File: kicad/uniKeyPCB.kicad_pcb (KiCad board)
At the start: 2 copper layers, 94 x 94 mm, 160 parts, among them J1 Conn_01x03_Socket, J2 Conn_01x03_Socket, J3 Conn_01x03_Socket, J4 Conn_01x03_Socket, J5 Conn_01x02_Socket, J6 Conn_01x02_Socket, J7 Conn_01x02_Socket, J8 Conn_01x02_Socket, SW1 SW_CHOC_HS, SW2 SW_MX_HS

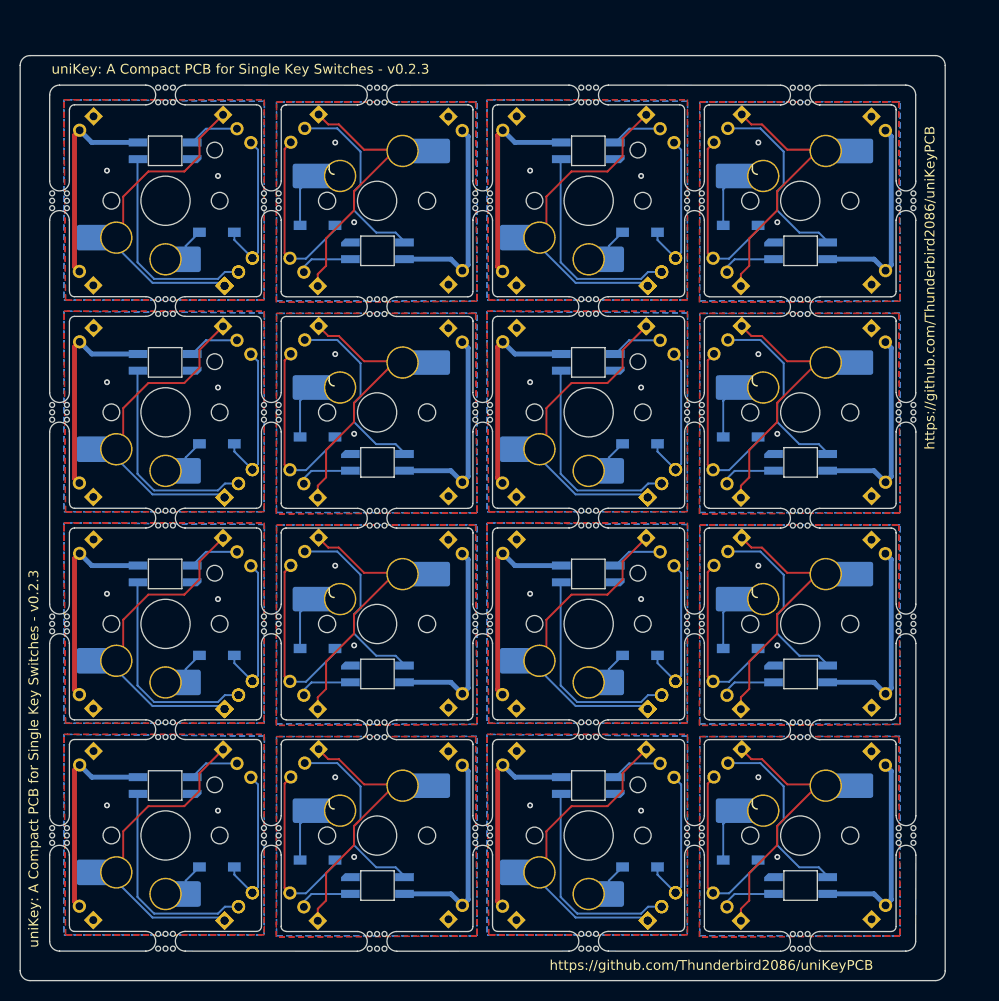
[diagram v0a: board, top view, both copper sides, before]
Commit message: more connectors
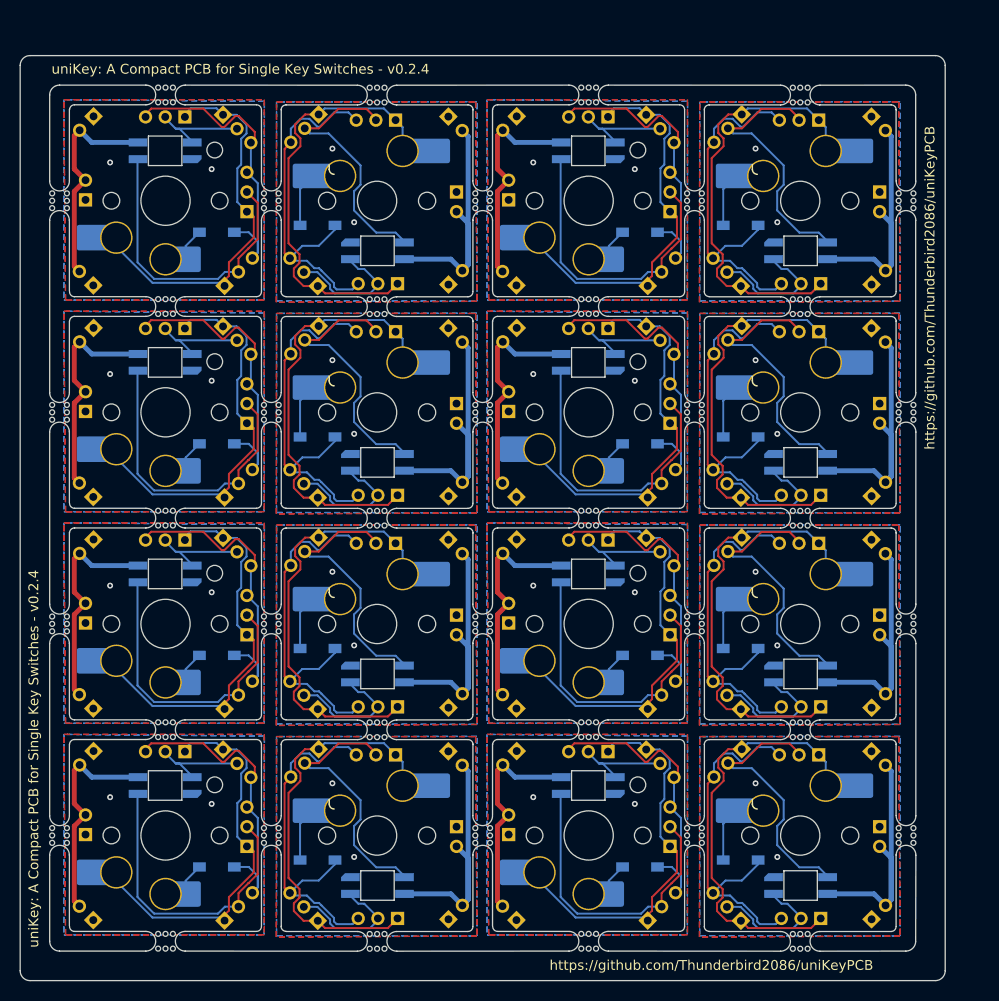
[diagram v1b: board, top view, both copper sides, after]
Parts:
- removed the J2 at (76.3, 136.0) (x2)
- removed the J2 at (119.3, 71.5) (x2)
- removed the J2 at (119.3, 114.5) (x2)
- removed the J2 at (76.3, 114.5) (x2)
- removed the J2 at (119.3, 136.0) (x2)
- removed the J2 at (76.3, 93.0) (x2)
- removed the J2 at (76.3, 71.5)
- removed the J2 at (119.3, 93.0) (x2)
- added J10: Conn_01x03_Socket, Connector_PinHeader_2.00mm:PinHeader_1x03_P2.00mm_Vertical, B.Cu at (121.6, 85.5)
- added J10: Conn_01x03_Socket, Connector_PinHeader_2.00mm:PinHeader_1x03_P2.00mm_Vertical, B.Cu at (121.6, 128.5)
- added J10: Conn_01x03_Socket, Connector_PinHeader_2.00mm:PinHeader_1x03_P2.00mm_Vertical, B.Cu at (78.6, 64.0)
- added J10: Conn_01x03_Socket, Connector_PinHeader_2.00mm:PinHeader_1x03_P2.00mm_Vertical, B.Cu at (78.6, 107.0)
- added J10: Conn_01x03_Socket, Connector_PinHeader_2.00mm:PinHeader_1x03_P2.00mm_Vertical, B.Cu at (121.6, 107.0)
- added J10: Conn_01x03_Socket, Connector_PinHeader_2.00mm:PinHeader_1x03_P2.00mm_Vertical, B.Cu at (78.6, 85.5)
- added J10: Conn_01x03_Socket, Connector_PinHeader_2.00mm:PinHeader_1x03_P2.00mm_Vertical, B.Cu at (121.6, 64.0)
- added J10: Conn_01x03_Socket, Connector_PinHeader_2.00mm:PinHeader_1x03_P2.00mm_Vertical, B.Cu at (78.6, 128.5)
- added J11: Conn_01x03_Socket, Connector_PinHeader_2.00mm:PinHeader_1x03_P2.00mm_Vertical, B.Cu at (93.9, 92.8)
- added J11: Conn_01x03_Socket, Connector_PinHeader_2.00mm:PinHeader_1x03_P2.00mm_Vertical, B.Cu at (93.9, 114.3)
- added J11: Conn_01x03_Socket, Connector_PinHeader_2.00mm:PinHeader_1x03_P2.00mm_Vertical, B.Cu at (136.9, 135.8)
- added J11: Conn_01x03_Socket, Connector_PinHeader_2.00mm:PinHeader_1x03_P2.00mm_Vertical, B.Cu at (136.9, 92.8)
- added J11: Conn_01x03_Socket, Connector_PinHeader_2.00mm:PinHeader_1x03_P2.00mm_Vertical, B.Cu at (93.9, 71.3)
- added J11: Conn_01x03_Socket, Connector_PinHeader_2.00mm:PinHeader_1x03_P2.00mm_Vertical, B.Cu at (93.9, 135.8)
- added J11: Conn_01x03_Socket, Connector_PinHeader_2.00mm:PinHeader_1x03_P2.00mm_Vertical, B.Cu at (136.9, 71.3)
- added J11: Conn_01x03_Socket, Connector_PinHeader_2.00mm:PinHeader_1x03_P2.00mm_Vertical, B.Cu at (136.9, 114.3)
- added J12: Conn_01x03_Socket, Connector_PinHeader_2.00mm:PinHeader_1x03_P2.00mm_Vertical, B.Cu at (93.7, 76.2)
- added J12: Conn_01x03_Socket, Connector_PinHeader_2.00mm:PinHeader_1x03_P2.00mm_Vertical, B.Cu at (93.7, 54.7)
- added J12: Conn_01x03_Socket, Connector_PinHeader_2.00mm:PinHeader_1x03_P2.00mm_Vertical, B.Cu at (136.7, 119.2)
- added J12: Conn_01x03_Socket, Connector_PinHeader_2.00mm:PinHeader_1x03_P2.00mm_Vertical, B.Cu at (136.7, 76.2)
- added J12: Conn_01x03_Socket, Connector_PinHeader_2.00mm:PinHeader_1x03_P2.00mm_Vertical, B.Cu at (93.7, 119.2)
- added J12: Conn_01x03_Socket, Connector_PinHeader_2.00mm:PinHeader_1x03_P2.00mm_Vertical, B.Cu at (93.7, 97.7)
- added J12: Conn_01x03_Socket, Connector_PinHeader_2.00mm:PinHeader_1x03_P2.00mm_Vertical, B.Cu at (136.7, 97.7)
- added J12: Conn_01x03_Socket, Connector_PinHeader_2.00mm:PinHeader_1x03_P2.00mm_Vertical, B.Cu at (136.7, 54.7)
- added J13: Conn_01x02_Socket, Connector_PinSocket_2.00mm:PinSocket_1x02_P2.00mm_Vertical, B.Cu at (142.9, 126.5)
- added J13: Conn_01x02_Socket, Connector_PinSocket_2.00mm:PinSocket_1x02_P2.00mm_Vertical, B.Cu at (99.9, 62.0)
- added J13: Conn_01x02_Socket, Connector_PinSocket_2.00mm:PinSocket_1x02_P2.00mm_Vertical, B.Cu at (99.9, 83.5)
- added J13: Conn_01x02_Socket, Connector_PinSocket_2.00mm:PinSocket_1x02_P2.00mm_Vertical, B.Cu at (142.9, 105.0)
- added J13: Conn_01x02_Socket, Connector_PinSocket_2.00mm:PinSocket_1x02_P2.00mm_Vertical, B.Cu at (142.9, 62.0)
- added J13: Conn_01x02_Socket, Connector_PinSocket_2.00mm:PinSocket_1x02_P2.00mm_Vertical, B.Cu at (99.9, 126.5)
- added J13: Conn_01x02_Socket, Connector_PinSocket_2.00mm:PinSocket_1x02_P2.00mm_Vertical, B.Cu at (99.9, 105.0)
- added J13: Conn_01x02_Socket, Connector_PinSocket_2.00mm:PinSocket_1x02_P2.00mm_Vertical, B.Cu at (142.9, 83.5)
- added J14: Conn_01x02_Socket, Connector_PinSocket_2.00mm:PinSocket_1x02_P2.00mm_Vertical, B.Cu at (62.2, 105.8)
- added J14: Conn_01x02_Socket, Connector_PinSocket_2.00mm:PinSocket_1x02_P2.00mm_Vertical, B.Cu at (105.2, 84.3)
- added J14: Conn_01x02_Socket, Connector_PinSocket_2.00mm:PinSocket_1x02_P2.00mm_Vertical, B.Cu at (105.2, 105.8)
- added J14: Conn_01x02_Socket, Connector_PinSocket_2.00mm:PinSocket_1x02_P2.00mm_Vertical, B.Cu at (62.2, 84.3)
- added J14: Conn_01x02_Socket, Connector_PinSocket_2.00mm:PinSocket_1x02_P2.00mm_Vertical, B.Cu at (105.2, 127.3)
- added J14: Conn_01x02_Socket, Connector_PinSocket_2.00mm:PinSocket_1x02_P2.00mm_Vertical, B.Cu at (105.2, 62.8)
- added J14: Conn_01x02_Socket, Connector_PinSocket_2.00mm:PinSocket_1x02_P2.00mm_Vertical, B.Cu at (62.2, 62.8)
- added J14: Conn_01x02_Socket, Connector_PinSocket_2.00mm:PinSocket_1x02_P2.00mm_Vertical, B.Cu at (62.2, 127.3)
- added J2: Conn_01x03_Socket, Connector_PinHeader_2.00mm:PinHeader_1x03_P2.00mm_Vertical, B.Cu at (76.3, 93.0)
- added J2: Conn_01x03_Socket, Connector_PinHeader_2.00mm:PinHeader_1x03_P2.00mm_Vertical, B.Cu at (119.3, 136.0)
- added J2: Conn_01x03_Socket, Connector_PinHeader_2.00mm:PinHeader_1x03_P2.00mm_Vertical, B.Cu at (119.3, 71.5)
- added J2: Conn_01x03_Socket, Connector_PinHeader_2.00mm:PinHeader_1x03_P2.00mm_Vertical, B.Cu at (76.3, 136.0)
- added J2: Conn_01x03_Socket, Connector_PinHeader_2.00mm:PinHeader_1x03_P2.00mm_Vertical, B.Cu at (119.3, 93.0)
- added J2: Conn_01x03_Socket, Connector_PinHeader_2.00mm:PinHeader_1x03_P2.00mm_Vertical, B.Cu at (119.3, 114.5)
- added J2: Conn_01x03_Socket, Connector_PinHeader_2.00mm:PinHeader_1x03_P2.00mm_Vertical, B.Cu at (76.3, 114.5)
- added J9: Conn_01x03_Socket, Connector_PinHeader_2.00mm:PinHeader_1x03_P2.00mm_Vertical, B.Cu at (115.3, 97.4)
- added J9: Conn_01x03_Socket, Connector_PinHeader_2.00mm:PinHeader_1x03_P2.00mm_Vertical, B.Cu at (72.3, 75.9)
- added J9: Conn_01x03_Socket, Connector_PinHeader_2.00mm:PinHeader_1x03_P2.00mm_Vertical, B.Cu at (115.3, 118.9)
- added J9: Conn_01x03_Socket, Connector_PinHeader_2.00mm:PinHeader_1x03_P2.00mm_Vertical, B.Cu at (115.3, 54.4)
- added J9: Conn_01x03_Socket, Connector_PinHeader_2.00mm:PinHeader_1x03_P2.00mm_Vertical, B.Cu at (72.3, 118.9)
- added J9: Conn_01x03_Socket, Connector_PinHeader_2.00mm:PinHeader_1x03_P2.00mm_Vertical, B.Cu at (72.3, 97.4)
- added J9: Conn_01x03_Socket, Connector_PinHeader_2.00mm:PinHeader_1x03_P2.00mm_Vertical, B.Cu at (72.3, 54.4)
- added J9: Conn_01x03_Socket, Connector_PinHeader_2.00mm:PinHeader_1x03_P2.00mm_Vertical, B.Cu at (115.3, 75.9)
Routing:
- net row1: track 148.0 -> 295.6 mm
- net col1: track 214.9 -> 346.6 mm
- net row0: track 125.2 -> 251.6 mm
- net LED0_out: track 173.4 -> 248.5 mm
- net LED1_in: track 40.3 -> 107.3 mm
- net col0: track 242.3 -> 307.1 mm
- net LED1_out: track 154.7 -> 217.9 mm
- net VCC: track 338.5 -> 399.9 mm
- net LED0_in: track 41.0 -> 80.3 mm
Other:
- board text added: "din"
- board text added: "dout"
- board text added: "row"
- board text added: "uniKey: A Compact PCB for Single Key Switches - v0.2.4"
- board text added: "v0.2.4"
- board text removed: "<- VCC ->"
- board text removed: "<- row ->"
- board text removed: "in"
- board text removed: "out"
- board text removed: "uniKey: A Compact PCB for Single Key Switches - v0.2.3"
- board text removed: "v0.2.3"

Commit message: Revert "more connectors (#4)"
This reverts commit e986b9c313ce46b497b00528d1270ea63e1c5e11.
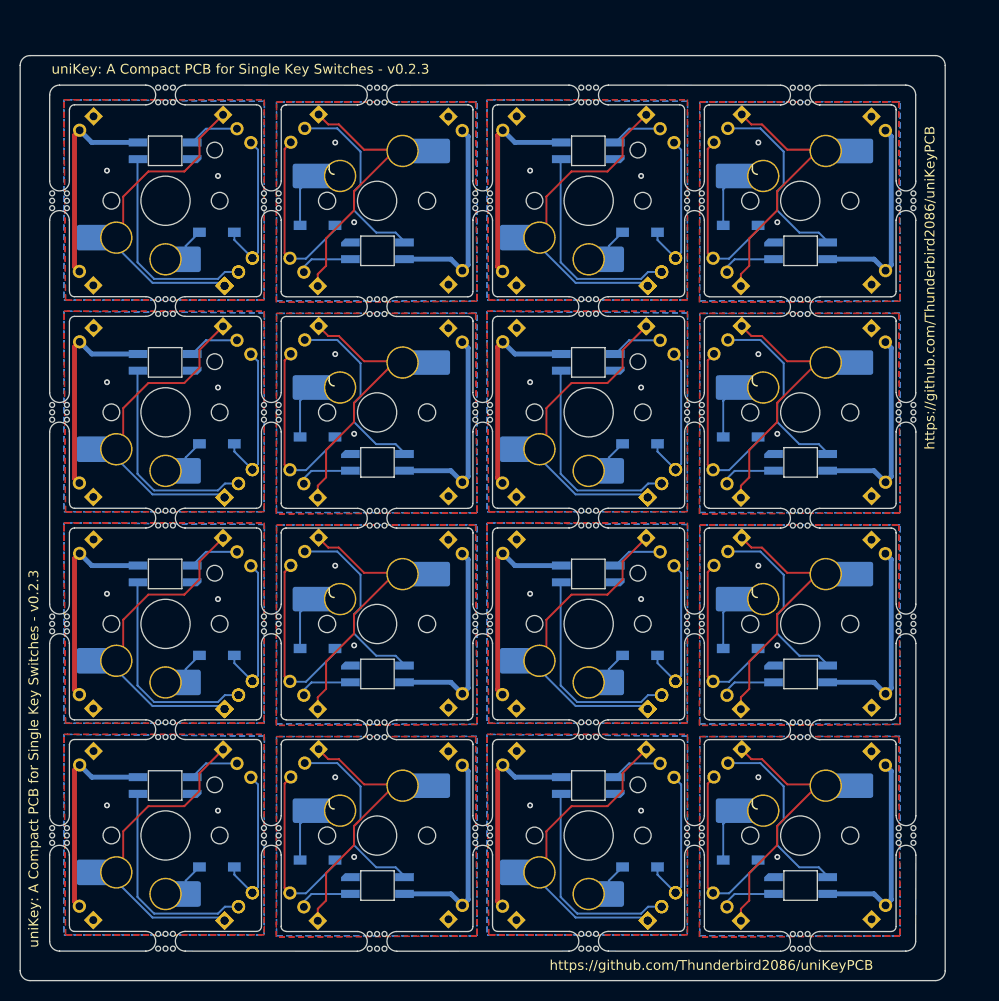
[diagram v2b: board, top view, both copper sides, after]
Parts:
- removed J10 (x8), J11 (x8), J12 (x8), J9 (x8): Conn_01x03_Socket, Connector_PinHeader_2.00mm:PinHeader_1x03_P2.00mm_Vertical
- removed J13 (x8), J14 (x8): Conn_01x02_Socket, Connector_PinSocket_2.00mm:PinSocket_1x02_P2.00mm_Vertical
- removed the J2 at (76.3, 93.0)
- removed the J2 at (119.3, 136.0)
- removed the J2 at (119.3, 71.5)
- removed the J2 at (76.3, 136.0)
- removed the J2 at (119.3, 93.0)
- removed the J2 at (119.3, 114.5)
- removed the J2 at (76.3, 114.5)
- added J2 (x2): Conn_01x03_Socket, Connector_PinHeader_2.00mm:PinHeader_1x03_P2.00mm_Vertical, B.Cu at (76.3, 136.0)
- added J2 (x2): Conn_01x03_Socket, Connector_PinHeader_2.00mm:PinHeader_1x03_P2.00mm_Vertical, B.Cu at (119.3, 71.5)
- added J2 (x2): Conn_01x03_Socket, Connector_PinHeader_2.00mm:PinHeader_1x03_P2.00mm_Vertical, B.Cu at (119.3, 114.5)
- added J2 (x2): Conn_01x03_Socket, Connector_PinHeader_2.00mm:PinHeader_1x03_P2.00mm_Vertical, B.Cu at (76.3, 114.5)
- added J2 (x2): Conn_01x03_Socket, Connector_PinHeader_2.00mm:PinHeader_1x03_P2.00mm_Vertical, B.Cu at (119.3, 136.0)
- added J2 (x2): Conn_01x03_Socket, Connector_PinHeader_2.00mm:PinHeader_1x03_P2.00mm_Vertical, B.Cu at (76.3, 93.0)
- added J2: Conn_01x03_Socket, Connector_PinHeader_2.00mm:PinHeader_1x03_P2.00mm_Vertical, B.Cu at (76.3, 71.5)
- added J2 (x2): Conn_01x03_Socket, Connector_PinHeader_2.00mm:PinHeader_1x03_P2.00mm_Vertical, B.Cu at (119.3, 93.0)
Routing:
- net row1: track 295.6 -> 148.0 mm
- net col1: track 346.6 -> 214.9 mm
- net row0: track 251.6 -> 125.2 mm
- net LED0_out: track 248.5 -> 173.4 mm
- net LED1_in: track 107.3 -> 40.3 mm
- net col0: track 307.1 -> 242.3 mm
- net LED1_out: track 217.9 -> 154.7 mm
- net VCC: track 399.9 -> 338.5 mm
- net LED0_in: track 80.3 -> 41.0 mm
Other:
- board text added: "<- VCC ->"
- board text added: "<- row ->"
- board text added: "in"
- board text added: "out"
- board text added: "uniKey: A Compact PCB for Single Key Switches - v0.2.3"
- board text added: "v0.2.3"
- board text removed: "din"
- board text removed: "dout"
- board text removed: "row"
- board text removed: "uniKey: A Compact PCB for Single Key Switches - v0.2.4"
- board text removed: "v0.2.4"
